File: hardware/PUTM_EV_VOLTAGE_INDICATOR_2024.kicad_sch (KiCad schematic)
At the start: 10 parts, among them J1 WIRE, J2 WIRE, J3 SCREW_TERMINAL, J4 SCREW_TERMINAL, J5 SCREW_TERMINAL, J6 SCREW_TERMINAL, J7 WIRE, J8 WIRE

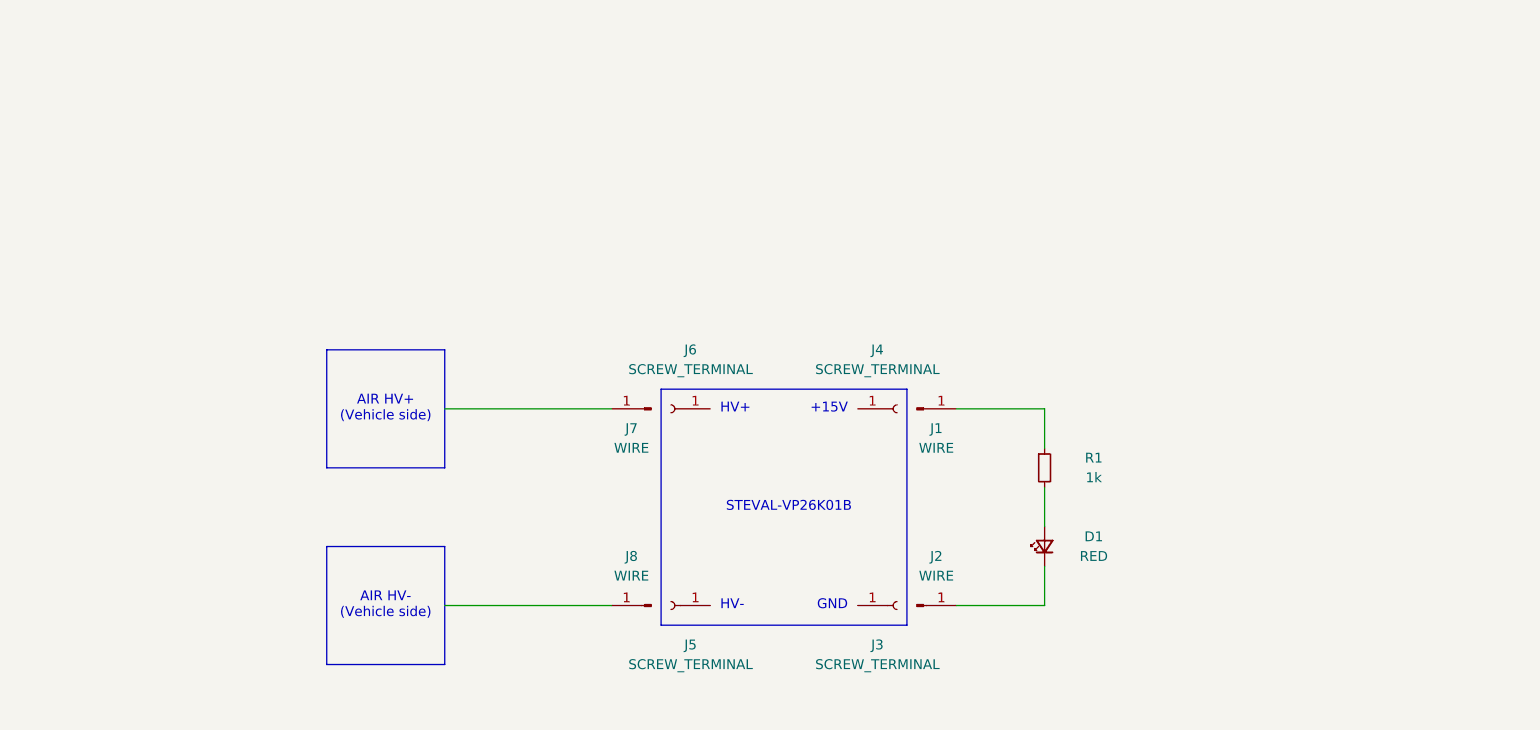
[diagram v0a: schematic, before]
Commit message: schematic updated
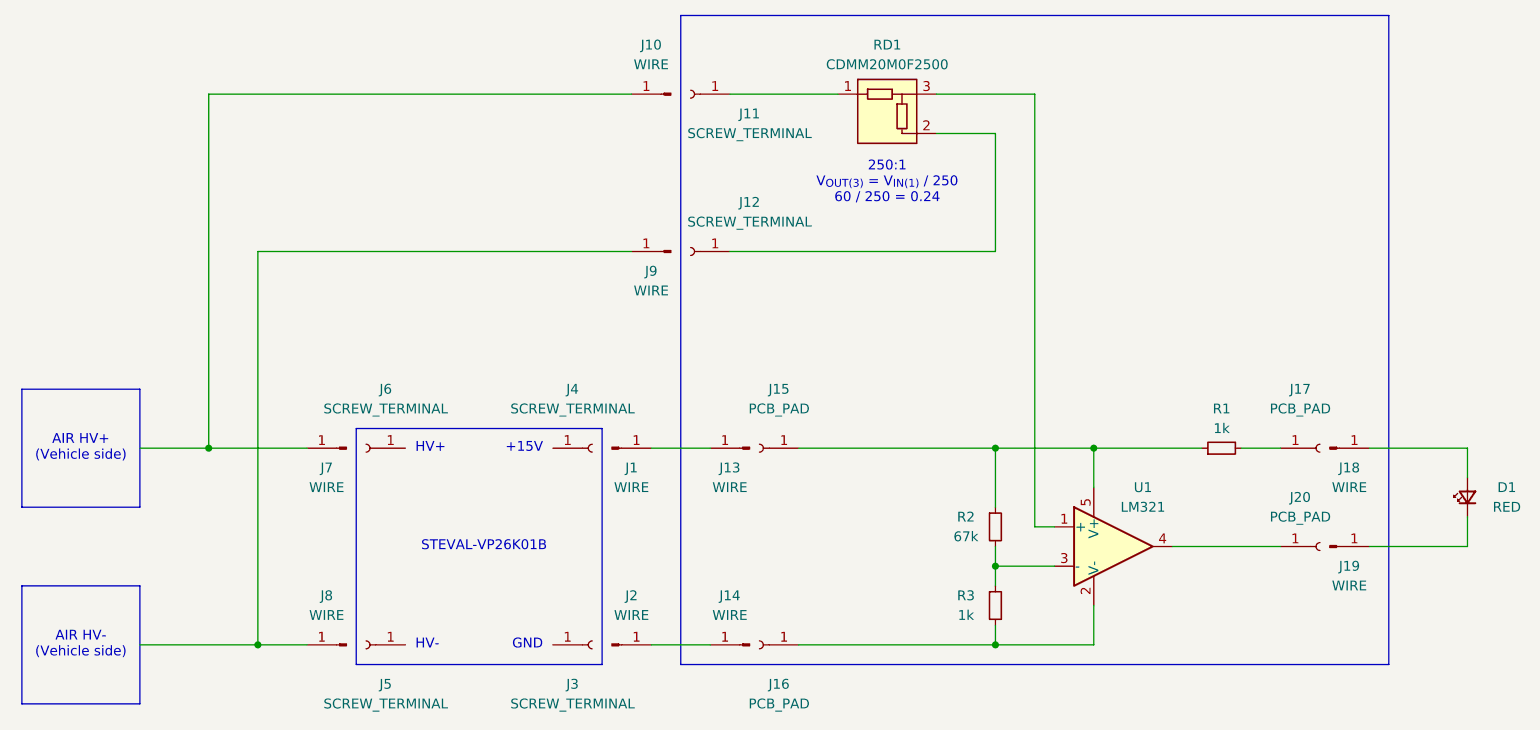
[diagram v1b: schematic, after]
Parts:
- added J10, J13, J14, J18, J19, J9: WIRE, symbol Connector:Conn_01x01_Pin
- added J11, J12: SCREW_TERMINAL, symbol Connector:Conn_01x01_Socket
- added J15, J16, J17, J20: PCB_PAD, symbol Connector:Conn_01x01_Socket
- added R2: 67k, symbol Device:R_Small
- added R3: 1k, symbol Device:R_Small
- added RD1: CDMM20M0F2500, CDMM:CDMM, symbol CDMM:CDMM2M50D4000DET
- added U1: LM321, Package_TO_SOT_SMD:SOT-23-5, symbol Amplifier_Operational:LM321
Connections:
- net at R1.1: now also J15.1 (Pin_1), R2.1, U1.5 (V+); no longer J1.1 (Pin_1)
- net at J7.1 (Pin_1): now also J10.1 (Pin_1)
- net at R1.2: now also J17.1 (Pin_1); no longer D1.2 (A)
- net at J2.1 (Pin_1): now also J14.1 (Pin_1); no longer D1.1 (K)
- net at J8.1 (Pin_1): now also J9.1 (Pin_1)
- new net: RD1.3, U1.1 (+)
- new net: J16.1 (Pin_1), R3.2, U1.2 (V-)
- new net: R2.2, R3.1, U1.3 (-)
- new net: J20.1 (Pin_1), U1.4
- new net: J1.1 (Pin_1), J13.1 (Pin_1)
- new net: J11.1 (Pin_1), RD1.1
- new net: J12.1 (Pin_1), RD1.2
- new net: D1.1 (K), J19.1 (Pin_1)
- new net: D1.2 (A), J18.1 (Pin_1)
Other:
- note added: "250:1 V_{OUT(3)} = V_{IN(1)} / 250 60 / 250 = 0.24"
- moved on the sheet: D1, J1, J2, J3, J4, J5, J6, J7, J8, R1
